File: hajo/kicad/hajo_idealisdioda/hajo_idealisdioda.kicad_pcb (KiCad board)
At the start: 2 copper layers, 51.1 x 80 mm, 16 parts, among them J1 LEDs, J2 Control, J3 Light switch, U1 LTC4355

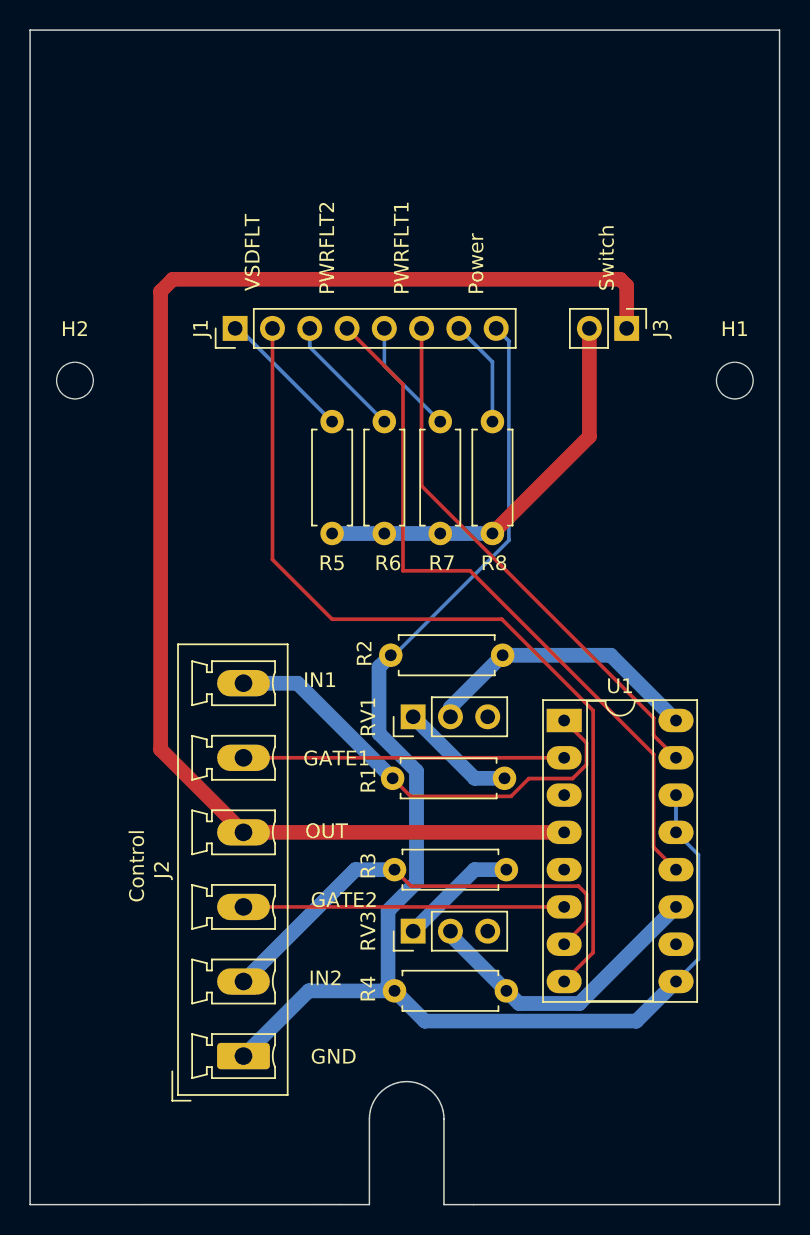
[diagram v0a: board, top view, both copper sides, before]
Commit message: fix boards
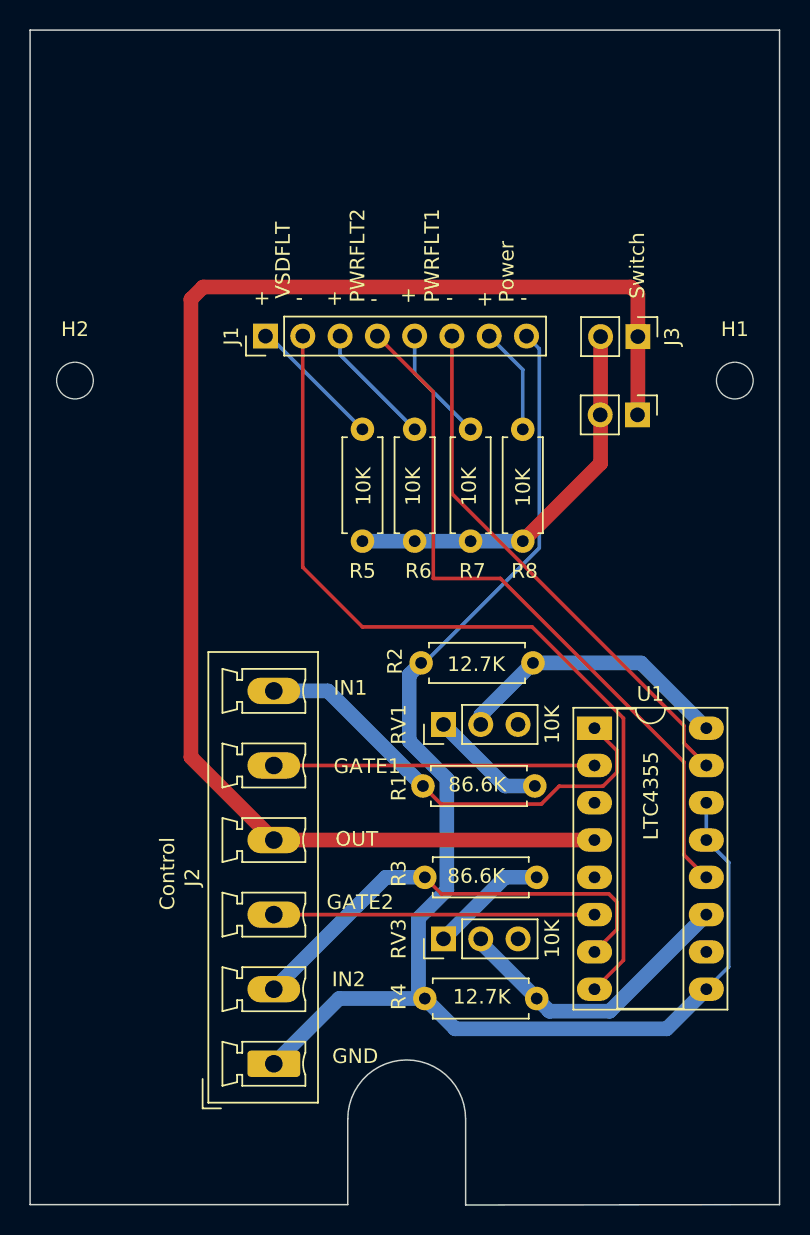
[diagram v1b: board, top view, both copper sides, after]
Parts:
- added J4: Light switch, Connector_PinHeader_2.54mm:PinHeader_1x02_P2.54mm_Vertical, F.Cu at (54.4, 39.2)
- moved R2 2.13 mm to (47.3, 56.1)
- moved R3 2.13 mm to (47.5, 70.7)
- moved R4 2.13 mm to (47.5, 79.0)
- moved R6 2.13 mm to (39.2, 47.8)
- moved R7 2.13 mm to (43.0, 47.8)
- moved R8 2.13 mm to (46.6, 47.8)
- moved J2 2.13 mm to (29.6, 83.4)
- moved J1 2.13 mm to (29.0, 33.8)
- moved R1 2.13 mm to (47.4, 64.5)
- moved R5 2.13 mm to (35.6, 47.8)
- moved RV3 2.13 mm to (41.2, 74.9)
- moved U1 2.13 mm to (51.4, 60.6)
- moved RV1 2.13 mm to (41.2, 60.3)
- moved J3 0.94 mm to (54.4, 33.9)
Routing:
- net Net-(J2-Pin_4): track 96.2 -> 100.3 mm
- net Net-(J3-Pin_2): track 27.6 -> 27.1 mm
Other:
- outline, holes or cut-outs redrawn
- board text added: "+"
- board text added: "-"
